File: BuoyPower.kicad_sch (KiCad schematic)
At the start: 14 parts

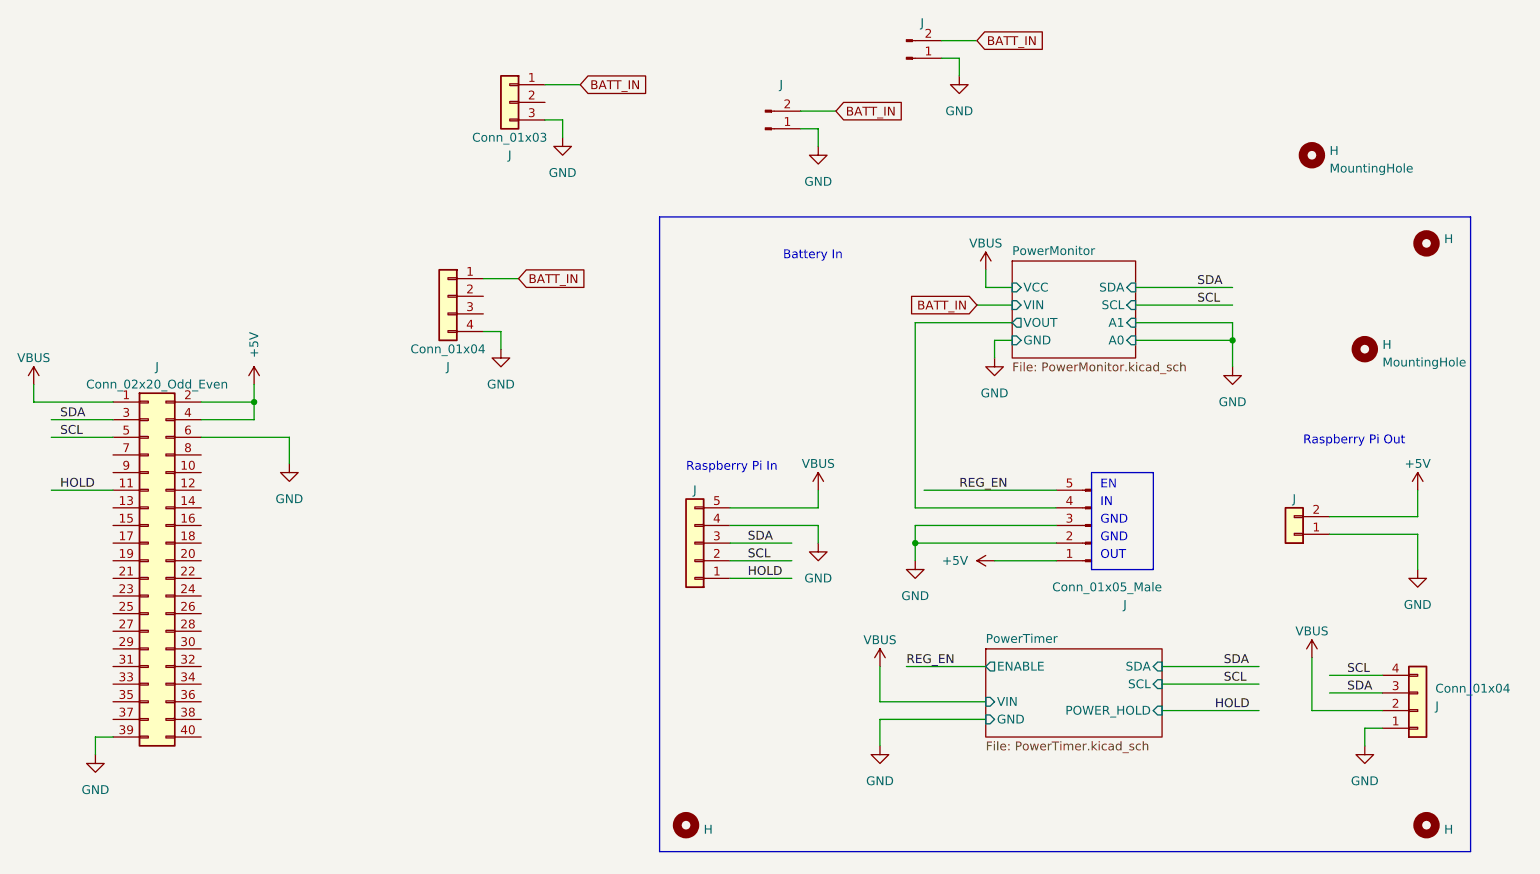
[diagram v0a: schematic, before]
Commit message: Ready to order.
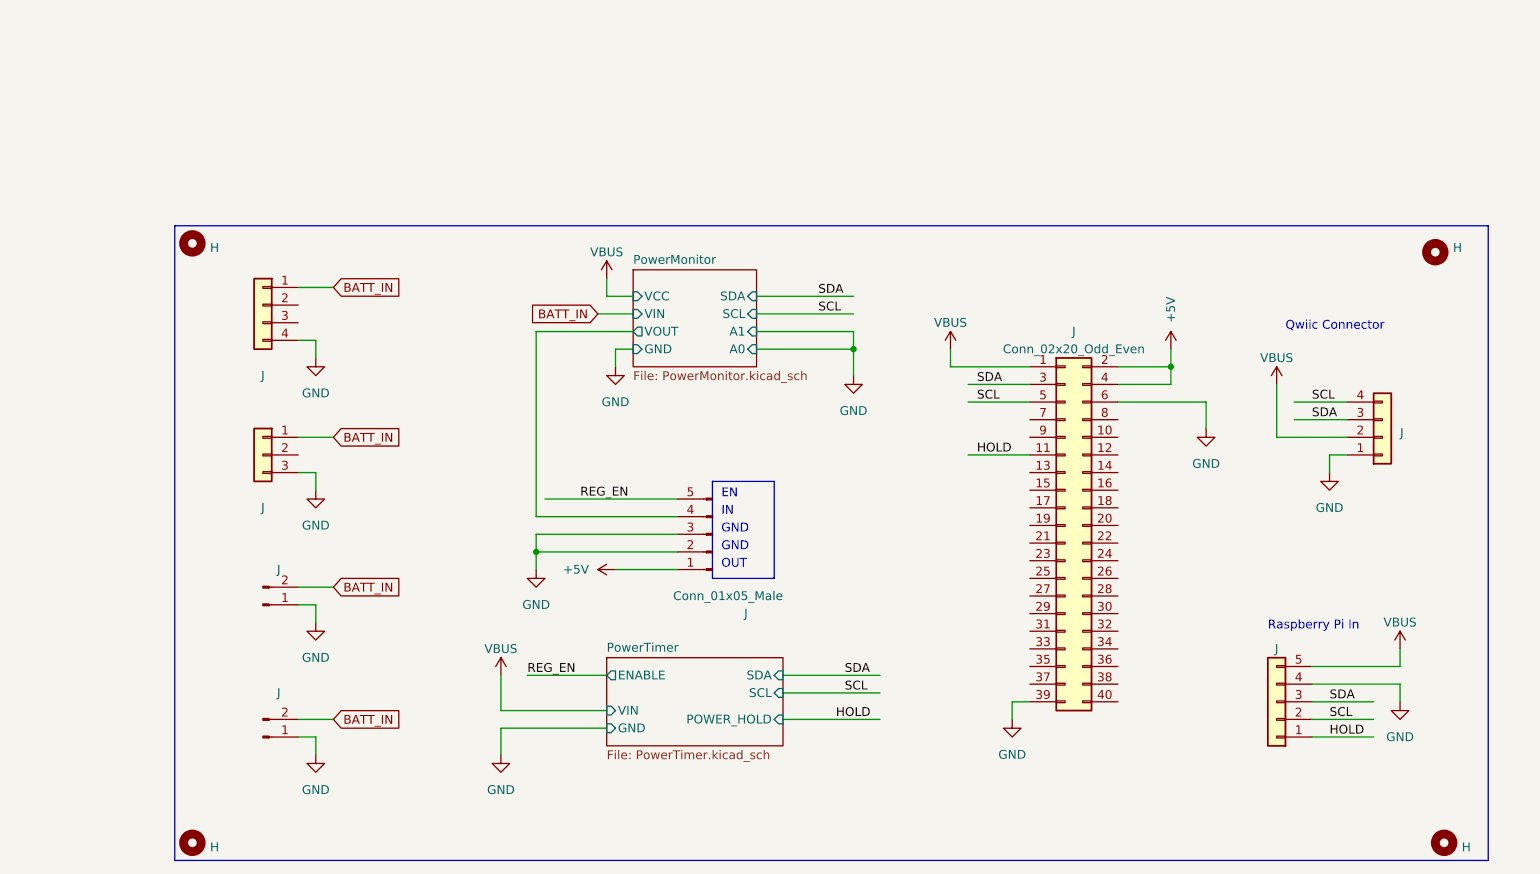
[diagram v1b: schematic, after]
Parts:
- removed H: MountingHole, symbol Mechanical:MountingHole
- removed J: Conn_01x02, symbol Connector_Generic:Conn_01x02
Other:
- note added: "Qwiic Connector"
- note removed: "Battery In"
- note removed: "Raspberry Pi Out"
- moved on the sheet: H, J
